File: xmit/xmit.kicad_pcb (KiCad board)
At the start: 4 copper layers, 90 x 60 mm, 67 parts, among them J1 Conn_Coaxial, J2 Conn_01x02, J3 Conn_01x02, J4 Conn_01x02, J5 Conn_01x02, U1 74LVC1G66, U10 L7812, U11 SN74LVC1G04DBV, U12 74LVC1G66, U13 74LVC1G66, U2 74LVC1G66, U3 74LVC1G66, U4 74LVC1G66, U5 74LVC1G66, U6 74LVC1G66, U7 TPS7A20xxxDBV, U9 L7805

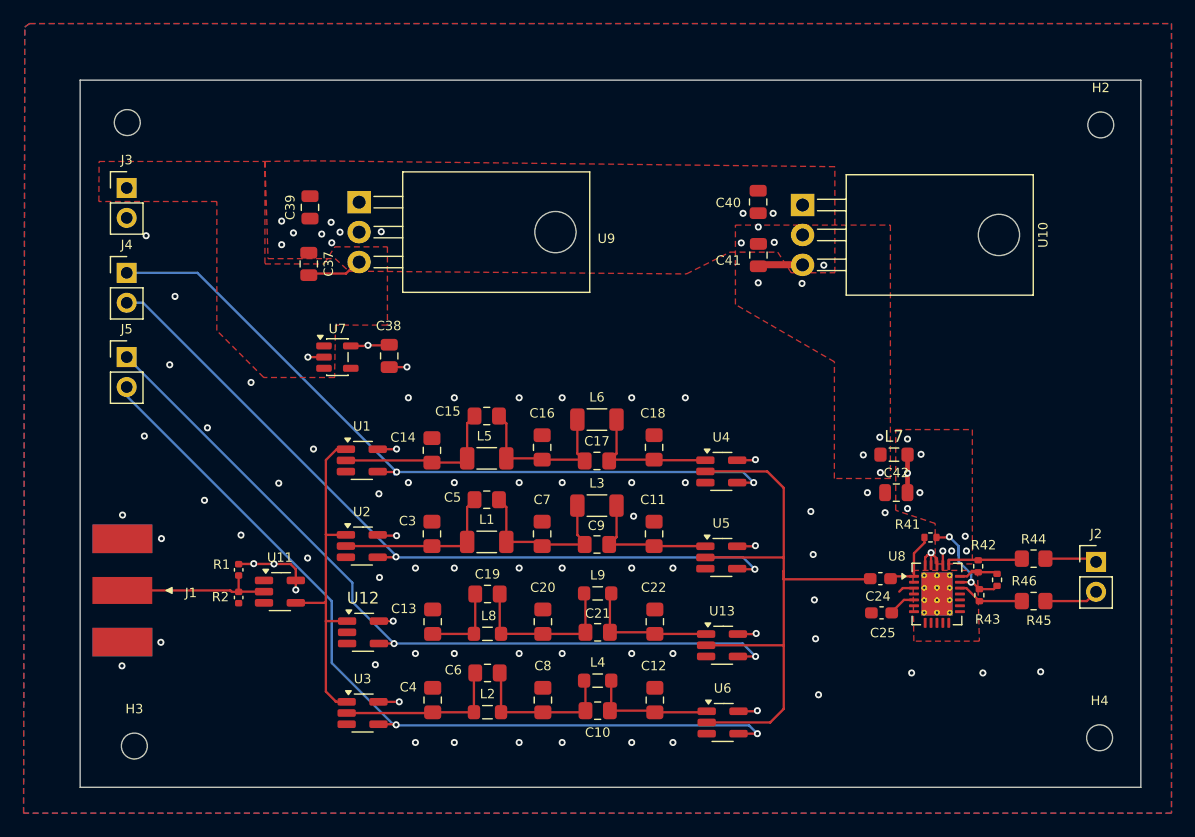
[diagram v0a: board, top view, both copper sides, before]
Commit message: Another WIP on transmitter layout. Should be pretty close.
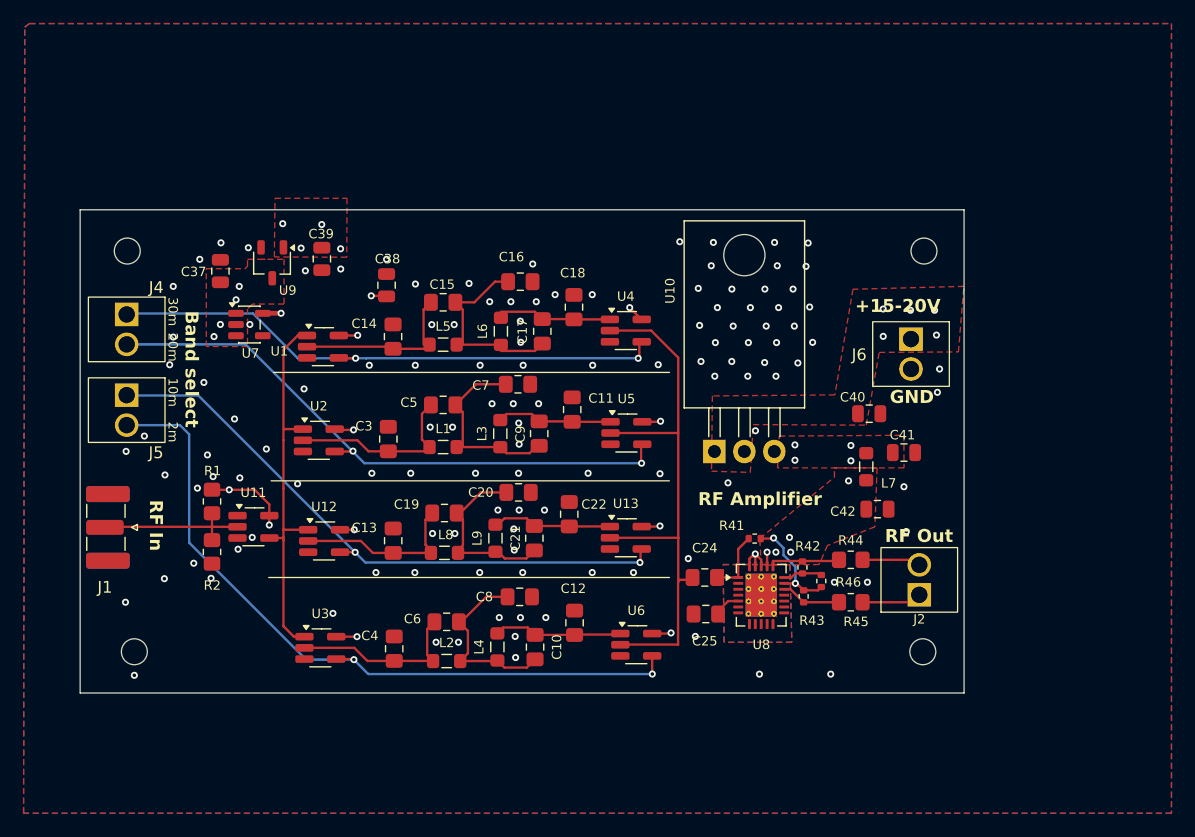
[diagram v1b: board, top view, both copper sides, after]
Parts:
- removed J3: Conn_01x02, Connector_PinHeader_2.54mm:PinHeader_1x02_P2.54mm_Vertical
- added J6: Conn_01x02, Connector:terminal_block_02, F.Cu at (200.5, 63.2)
- C24, C25: footprint Capacitor_SMD:C_0603_1608Metric_Pad1.08x0.95mm_HandSolder -> Capacitor_SMD:C_0805_2012Metric_Pad1.18x1.45mm_HandSolder
- J1: footprint Connector_Coaxial:SMA_Molex_73251-1153_EdgeMount_Horizontal -> Connector_Coaxial:SMA_Samtec_SMA-J-P-H-ST-EM1_EdgeMount
- J2, J4, J5: footprint Connector_PinHeader_2.54mm:PinHeader_1x02_P2.54mm_Vertical -> Connector:terminal_block_02
- L1, L3, L5, L6: footprint Inductor_SMD:L_1206_3216Metric_Pad1.22x1.90mm_HandSolder -> Inductor_SMD:L_0805_2012Metric_Pad1.05x1.20mm_HandSolder
- R1, R2: footprint Capacitor_SMD:C_0402_1005Metric -> Resistor_SMD:R_0805_2012Metric_Pad1.20x1.40mm_HandSolder
- U9: value L7805 -> TLV760; footprint Package_TO_SOT_THT:TO-220-3_Horizontal_TabDown -> Package_TO_SOT_SMD:TSOT-23
- moved U10 22.2 mm to (183.8, 71.5), turned to 0 degrees
- moved C41 20.8 mm to (199.9, 71.6), turned to 180 degrees
- moved C40 20.3 mm to (196.9, 68.3), turned to 180 degrees
- moved H2 18.4 mm to (201.6, 54.5)
- moved H4 16.7 mm to (201.5, 88.5)
- moved R44 15.5 mm to (195.4, 80.7)
- moved R45 15.5 mm to (195.4, 84.3)
- moved J2 15.1 mm to (201.2, 82.4), turned to 90 degrees
- moved R43 14.9 mm to (191.4, 83.8)
- moved R46 14.9 mm to (192.9, 82.5)
- moved C25 14.9 mm to (183.1, 85.3)
- moved R41 14.9 mm to (187.2, 78.9)
- moved R42 14.9 mm to (191.3, 81.3)
- moved U8 14.9 mm to (187.8, 83.7)
- moved C24 14.9 mm to (183.0, 82.2)
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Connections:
- J2 pad 1: out+ -> out-
- J2 pad 2: out- -> out+
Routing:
- net band.30m: track 63.9 -> 48.1 mm
- net band.10m: track 67.7 -> 52.0 mm
- net band.20m: track 65.9 -> 51.2 mm
- net band.2m: track 72.3 -> 61.8 mm
- net Net-(C13-Pad1): track 6.76 -> 15.1 mm
- net rf_drive: track 54.2 -> 49.1 mm
- net +5V: track 4.73 -> 0.00 mm, vias 0 -> 3
- net GND: track 7.71 -> 3.46 mm, vias 75 -> 125
- net /Power/raw12V: track 3.73 -> 0.00 mm, vias 6 -> 4
- net +12V: track 4.42 -> 1.20 mm, vias 9 -> 5
- net Net-(U1-Pad1): track 30.0 -> 33.1 mm
- net Net-(C5-Pad2): track 13.3 -> 16.1 mm
- net Net-(C10-Pad1): track 12.7 -> 15.3 mm
- net Net-(C15-Pad2): track 14.1 -> 16.6 mm
- net Net-(C19-Pad2): track 13.5 -> 15.6 mm
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- added copper zone on In2.Cu, net /Power/+20V
- added copper zone on In2.Cu, net GND
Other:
- board size 90 x 60 mm -> 75 x 41 mm
- board text added: "+15-20V"
- board text added: "10m"
- board text added: "20m"
- board text added: "2m"
- board text added: "30m"
- board text added: "Band select"
- board text added: "GND"
- board text added: "RF Amplifier"
- board text added: "RF In"
- board text added: "RF Out"
